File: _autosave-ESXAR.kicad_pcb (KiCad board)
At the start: 2 copper layers, 71.1 x 60.6 mm, 55 parts, among them P1 ANALOG, P10 USB_A, P11 USB_B, P12 SERVO/INPUT, P13 ANALOG, P16 BREADBOARD_POWER, P17 SENSOR, P18 EXTIO, P19 UNIVERSAL, P2 BREADBOARD, P20 UNIVERSAL, P3 PROGRAM, P4 OPAMP EX, P5 MODEJP, P6 VCCJP, P7 GNDJP, P8 SCREW, SW1 RESET, SW2 DIN, U1 ESP-WROOM-02, U2 NJM4556A, U3 AUDIO_JACK, U4 MT5201-3.3N, U5 TLP222A, U6 Mini360, U7 LD1117CV33, U8 TA48M033F

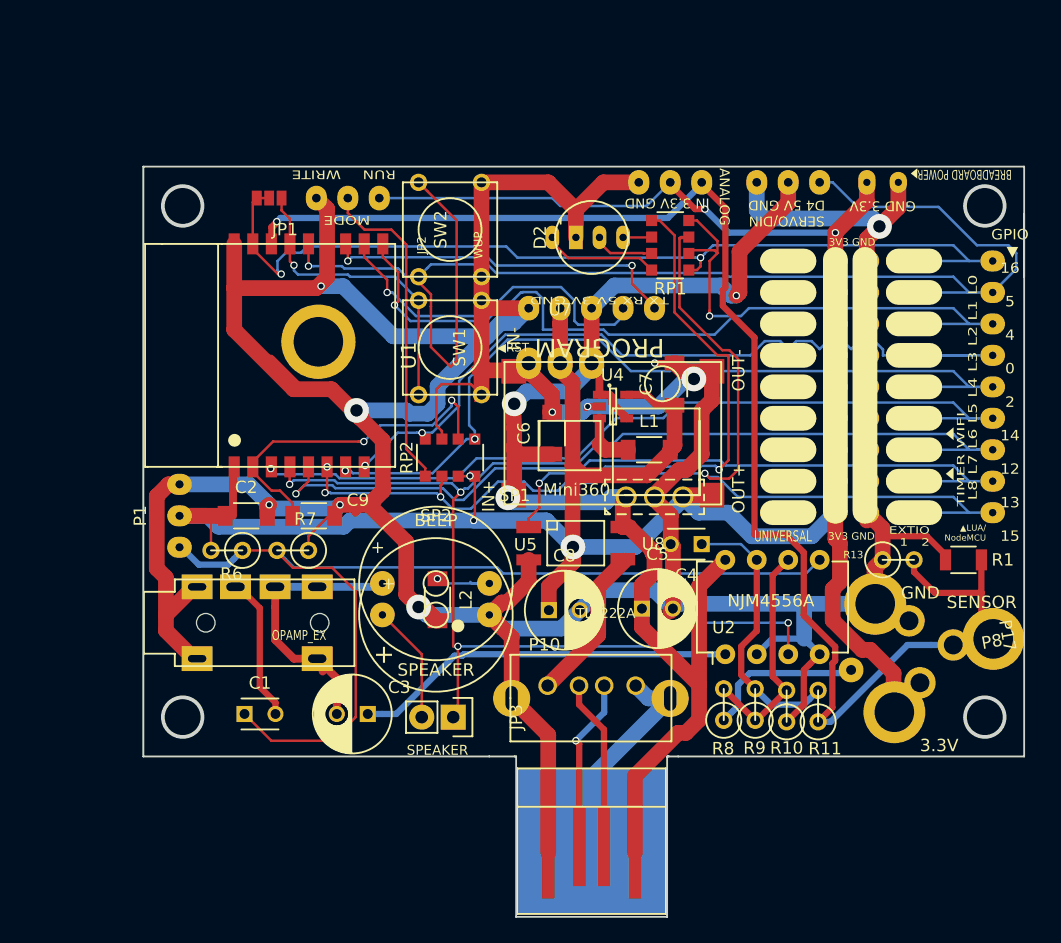
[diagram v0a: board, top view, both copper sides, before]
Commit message: Ver.20160805 change outline, rayout, delete opamp, etc...
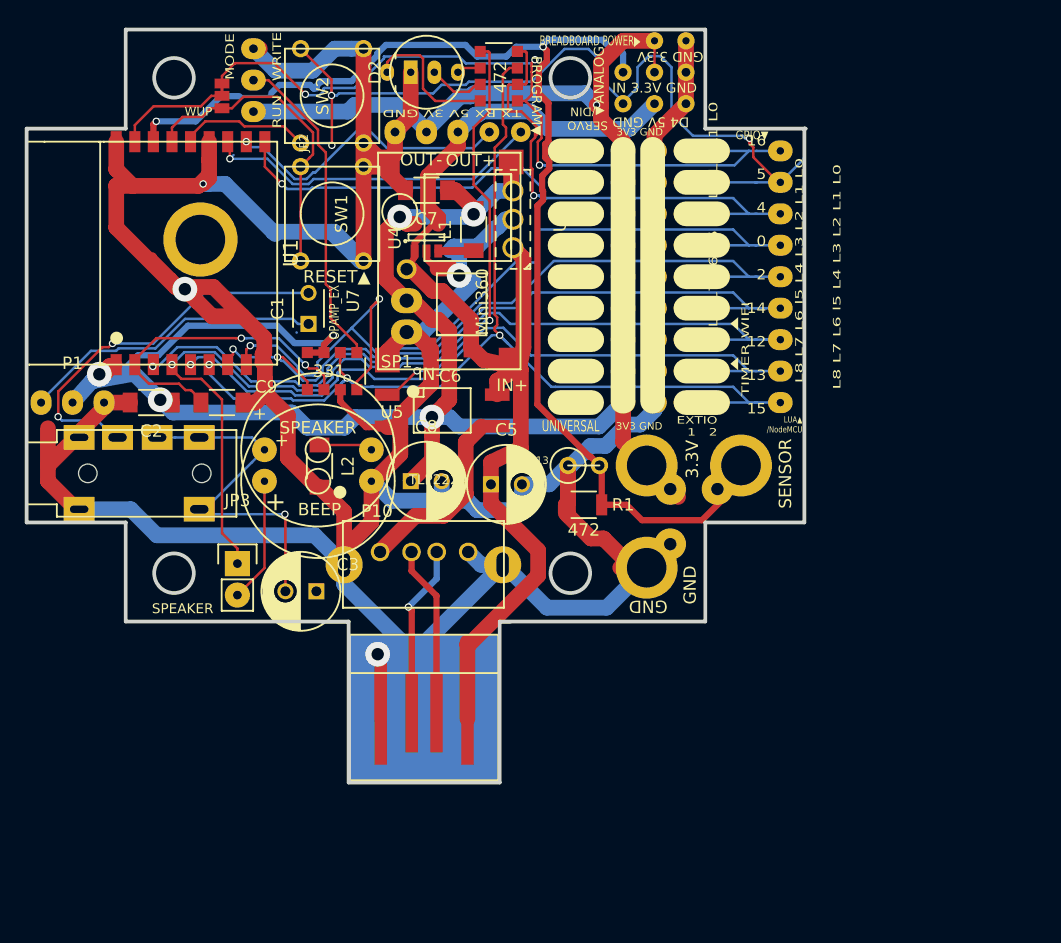
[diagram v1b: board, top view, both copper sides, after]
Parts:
- removed C4: 0.1uF, Capacitors_ThroughHole:C_Disc_D3_P2.5
- removed P4: OPAMP EX, Wire_Pads:SolderWirePad_single_0-8mmDrill
- removed R10, R11, R6, R7, R8, R9: 4.7kΩ, Discret:R1
- removed U2: NJM4556A, Housings_DIP:DIP-8_W7.62mm
- JP1, P17, P8: moved to B.Cu
- moved OSHW 35.6 mm to (132.1, 97.2)
- moved C1 31.9 mm to (149.9, 102.9), turned to 90 degrees
- moved R1 31.0 mm to (172.1, 117.5)
- moved R13 26.5 mm to (172.1, 114.3)
- moved C7 25.4 mm to (159.4, 92.1), turned to 180 degrees
- moved U8 25.2 mm to (166.4, 94.4), turned to 270 degrees
- moved L1 22.7 mm to (163.2, 95.2), turned to 90 degrees
- moved P8 21.8 mm to (184.8, 118.1), turned to 90 degrees
- moved JP3 21.4 mm to (144.1, 122.2), turned to 0 degrees
- moved P17 21.3 mm to (182.2, 119.4), turned to 90 degrees
- moved P16 20.6 mm to (179.1, 80.0)
- moved U4 20.3 mm to (159.4, 95.9), turned to 90 degrees
- moved RP1 19.4 mm to (165.2, 82.9)
- moved P18 19.3 mm to (182.9, 99.1)
- moved P20 19.3 mm to (172.7, 99.1)
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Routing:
- net Net-(C1-Pad1): track 82.6 -> 24.6 mm
- net GND: track 416.7 -> 376.2 mm, vias 10 -> 4
- net Net-(JP3-Pad1): track 117.6 -> 81.2 mm, vias 4 -> 1
- net Net-(C3-Pad1): track 30.9 -> 0.00 mm
- net Net-(P12-Pad1): track 111.5 -> 84.1 mm, vias 1 -> 3
- net Net-(C4-Pad1): track 22.5 -> 0.00 mm
- net +3V3: track 217.9 -> 196.6 mm, vias 6 -> 7
- net Net-(P13-Pad1): track 121.3 -> 100.5 mm, vias 1 -> 2
- net Net-(C1-Pad2): track 11.7 -> 31.0 mm, vias 0 -> 2
- net Net-(R10-Pad2): track 18.7 -> 0.00 mm
- net +5V: track 109.7 -> 92.5 mm, vias 3 -> 0
- net Net-(P4-Pad1): track 13.2 -> 0.00 mm
- net Net-(P18-Pad3): track 79.1 -> 69.1 mm
- net Net-(RP1-Pad5): track 43.0 -> 34.4 mm
- net Net-(P18-Pad8): track 67.4 -> 58.9 mm
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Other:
- board size 71.1 x 60.6 mm -> 62.9 x 60.9 mm
- board text added: "16 5 4 0 2 14 12 13 15"
- board text added: "331"
- board text added: "472"
- board text added: "D4 5V GND"
- board text added: "ESXAR Ver.20160816"
- board text added: "GPIO▼"
- board text added: "L8 L7 L6 l5 L4 L3 L2 L1 L0"
- board text added: "LUA▲ /NodeMCU"
- board text added: "PROGRAM▼"
- board text added: "RESET▲"
- board text added: "SERVO ◀/DIN"
- board text added: "▲BREADBOARD"
- board text added: "◀BREADBOARD POWER"
- board text removed: "ESXAR Ver.20160804"
- board text removed: "GPIO ▼ 16 5 4 0 2 14 12 13 15"
- board text removed: "PROGRAM"
- board text removed: "SERVO/DIN D4 5V GND"
- board text removed: "▲LUA/ NodeMCU"
- board text removed: "◀RST"
